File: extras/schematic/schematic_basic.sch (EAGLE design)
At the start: 18 parts, among them U1 SI4735-D60-GU

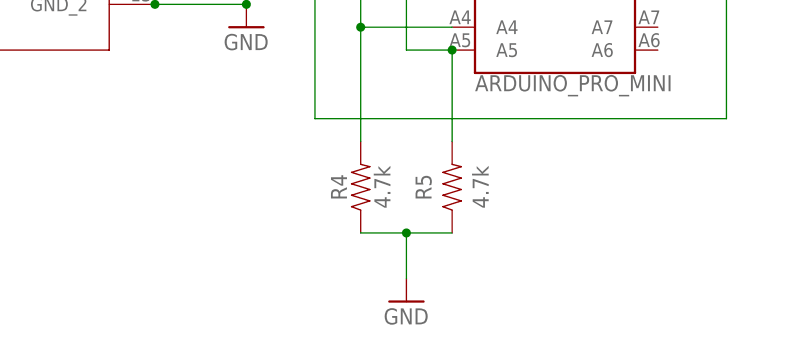
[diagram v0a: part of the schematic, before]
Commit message: SI47XX Arduino Library
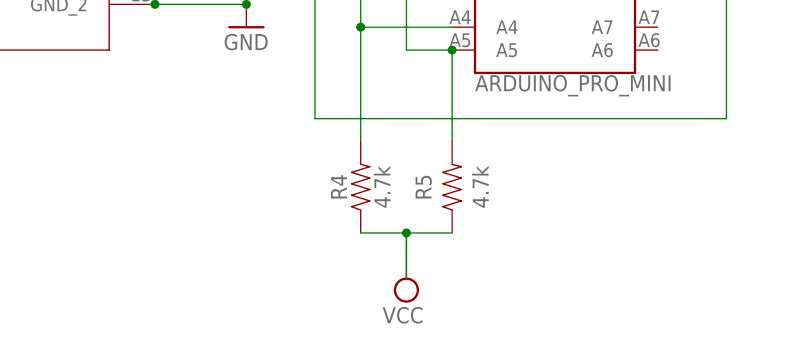
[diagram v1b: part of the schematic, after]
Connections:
- net GND: no longer R4.1, R5.1
- net VCC: now also R4.1, R5.1
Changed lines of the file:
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@@
 <part name="R4" library="SparkFun-Resistors" library_urn="urn:adsk.eagle:library:532" deviceset="4.7KOHM" device="-0603-1/10W-1%" package3d_urn="urn:adsk.eagle:package:39650/1" value="4.7k"/>
 <part name="R5" library="SparkFun-Resistors" library_urn="urn:adsk.eagle:library:532" deviceset="4.7KOHM" device="-0603-1/10W-1%" package3d_urn="urn:adsk.eagle:package:39650/1" value="4.7k"/>
-<part name="GND2" library="supply1" library_urn="urn:adsk.eagle:library:371" deviceset="GND" device=""/>
 <part name="SUPPLY1" library="supply2" library_urn="urn:adsk.eagle:library:372" deviceset="VCC" device=""/>
 <part name="C1" library="SparkFun-Capacitors" library_urn="urn:adsk.eagle:library:510" deviceset="22NF/22,000PF" device="-0603-50V-10%" package3d_urn="urn:adsk.eagle:package:37414/1" value="22nF"/>
@@
 <part name="SUPPLY2" library="supply2" library_urn="urn:adsk.eagle:library:372" deviceset="VCC" device=""/>
 <part name="GND7" library="supply1" library_urn="urn:adsk.eagle:library:371" deviceset="GND" device=""/>
+<part name="SUPPLY3" library="supply2" library_urn="urn:adsk.eagle:library:372" deviceset="VCC" device=""/>
 </parts>
 <sheets>
@@
 <attribute name="VALUE" x="70.104" y="68.58" size="1.778" layer="96" font="vector" rot="R270" align="top-center"/>
 </instance>
-<instance part="GND2" gate="1" x="60.96" y="55.88" smashed="yes">
-<attribute name="VALUE" x="58.42" y="53.34" size="1.778" layer="96"/>
-</instance>
 <instance part="SUPPLY1" gate="G$1" x="50.8" y="109.22" smashed="yes" rot="R270">
 <attribute name="VALUE" x="53.975" y="108.585" size="1.778" layer="96"/>
@@
 <instance part="GND7" gate="1" x="-58.42" y="86.36" smashed="yes">
 <attribute name="VALUE" x="-60.96" y="83.82" size="1.778" layer="96"/>
+</instance>
+<instance part="SUPPLY3" gate="G$1" x="60.96" y="58.42" smashed="yes" rot="R180">
+<attribute name="VALUE" x="62.865" y="55.245" size="1.778" layer="96" rot="R180"/>
 </instance>
 </instances>
@@
 <junction x="33.02" y="91.44"/>
 <junction x="33.02" y="96.52"/>
-</segment>
-<segment>
-<pinref part="R4" gate="G$1" pin="1"/>
-<pinref part="GND2" gate="1" pin="GND"/>
-<wire x1="55.88" y1="63.5" x2="60.96" y2="63.5" width="0.1524" layer="91"/>
-<wire x1="60.96" y1="63.5" x2="60.96" y2="58.42" width="0.1524" layer="91"/>
-<pinref part="R5" gate="G$1" pin="1"/>
-<wire x1="66.04" y1="63.5" x2="60.96" y2="63.5" width="0.1524" layer="91"/>
-<junction x="60.96" y="63.5"/>
 </segment>
 <segment>
@@
 <wire x1="101.6" y1="111.76" x2="101.6" y2="109.22" width="0.1524" layer="91"/>
 </segment>
-</net>
+<segment>
+<pinref part="R4" gate="G$1" pin="1"/>
+<wire x1="55.88" y1="63.5" x2="60.96" y2="63.5" width="0.1524" layer="91"/>
+<wire x1="60.96" y1="63.5" x2="60.96" y2="58.42" width="0.1524" layer="91"/>
+<pinref part="R5" gate="G$1" pin="1"/>
+<wire x1="66.04" y1="63.5" x2="60.96" y2="63.5" width="0.1524" layer="91"/>
+<junction x="60.96" y="63.5"/>
+<pinref part="SUPPLY3" gate="G$1" pin="VCC"/>
+<wire x1="60.96" y1="60.96" x2="60.96" y2="63.5" width="0.1524" layer="91"/>
+</segment>
+</net>
